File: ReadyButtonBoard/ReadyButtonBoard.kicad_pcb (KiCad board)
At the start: 2 copper layers, 41.9 x 44.5 mm, 7 parts, among them J2 Conn_01x02_Socket

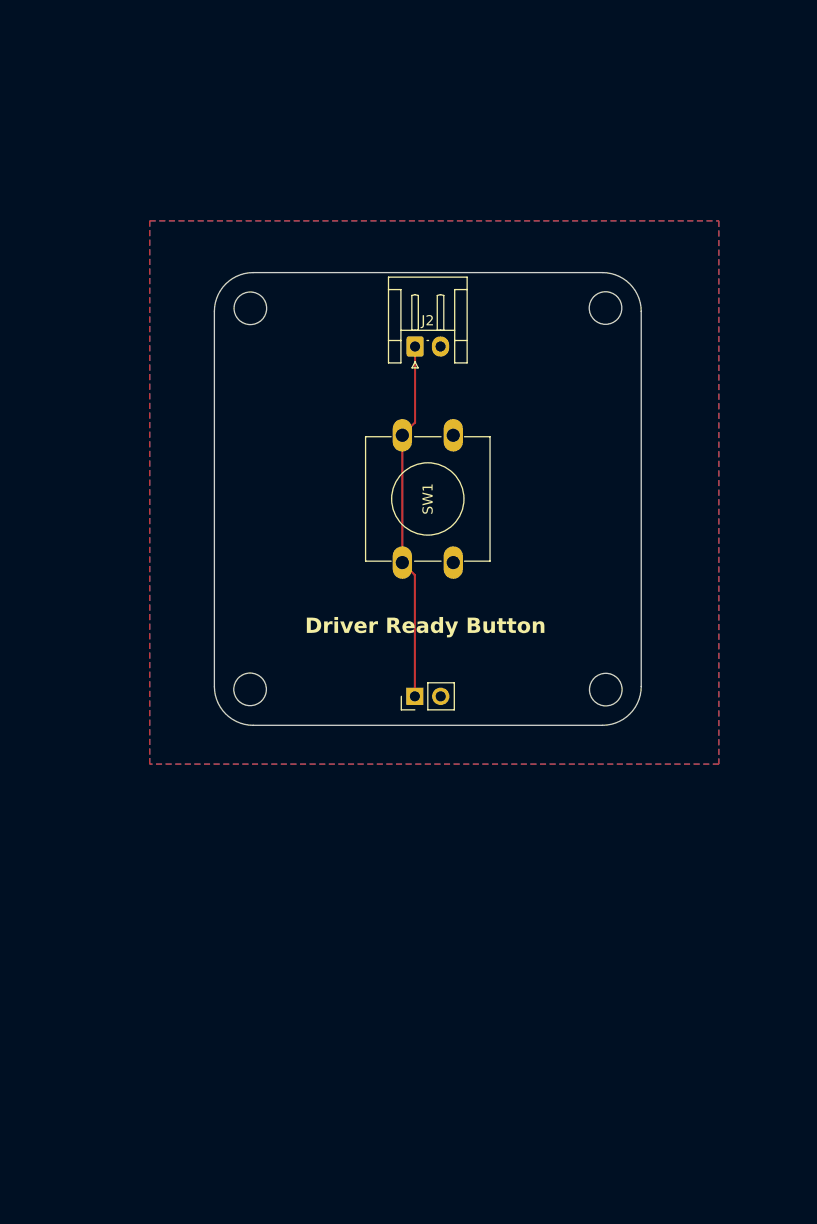
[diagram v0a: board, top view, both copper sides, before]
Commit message: finish ready button board and prod files
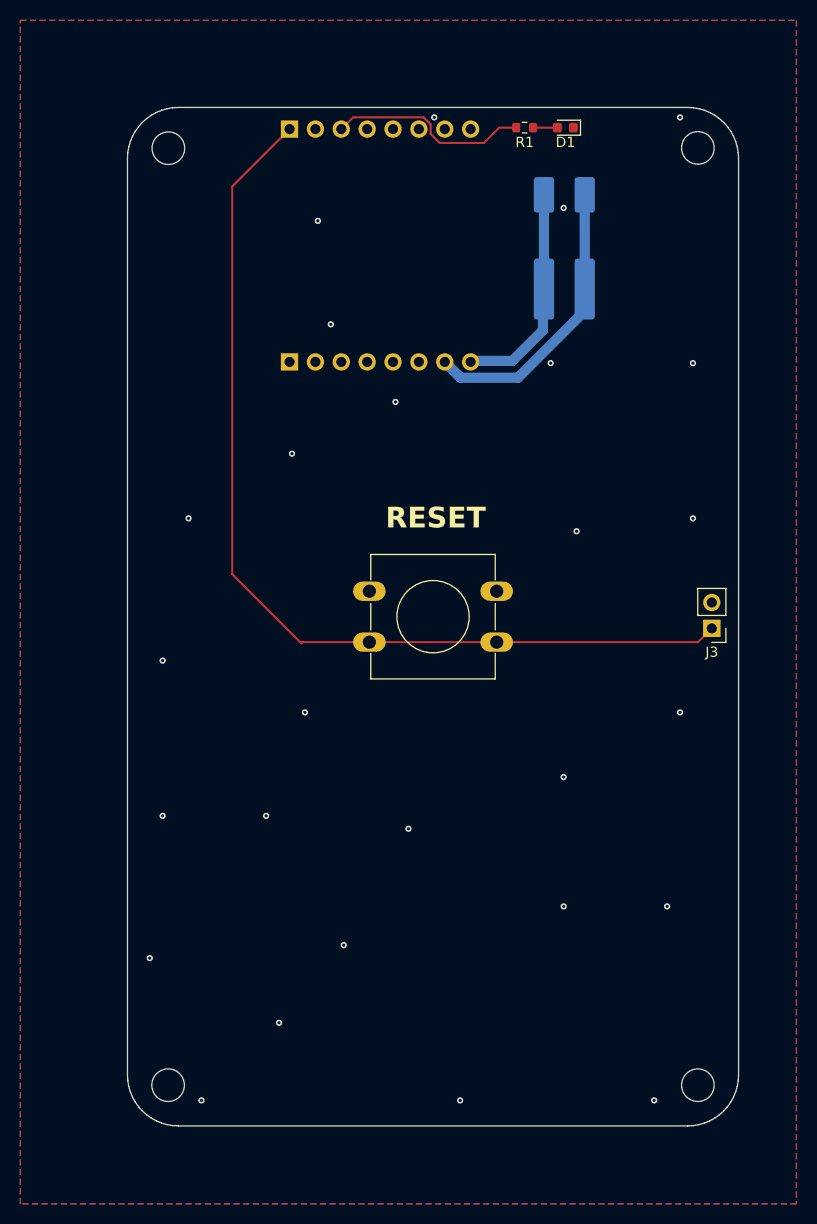
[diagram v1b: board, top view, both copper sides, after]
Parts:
- added D1: Red, LED_SMD:LED_0603_1608Metric, F.Cu at (164.0, 48.0)
- added J3: START, Connector_PinHeader_2.54mm:PinHeader_1x02_P2.54mm_Vertical, F.Cu at (178.4, 97.2)
- added J9: WAGO, WAGO_2060-452_998-404:2060-452_998-404, B.Cu at (163.9, 60.5)
- added R1: 470, Resistor_SMD:R_0603_1608Metric, F.Cu at (160.0, 48.0)
- J1: value ~ -> Conn_01x08_Socket; footprint Connector_PinHeader_2.54mm:PinHeader_1x02_P2.54mm_Vertical -> Connector_PinSocket_2.54mm:PinSocket_1x08_P2.54mm_Vertical; moved to B.Cu
- J2: value Conn_01x02_Socket -> Conn_01x08_Socket; footprint Connector_JST:JST_EH_S2B-EH_1x02_P2.50mm_Horizontal -> Connector_PinSocket_2.54mm:PinSocket_1x08_P2.54mm_Vertical; moved to B.Cu
- SW1: value ~ -> START
- moved J1 57.0 mm to (136.9, 48.1), turned to -90 degrees
- moved H4 39.9 mm to (177.0, 142.0)
- moved H3 39.7 mm to (125.0, 142.0)
- moved H2 18.1 mm to (177.0, 50.0)
- moved H1 17.7 mm to (125.0, 50.0)
- moved SW1 17.4 mm to (144.8, 93.5), turned to 0 degrees
- moved J2 12.4 mm to (136.9, 71.0), turned to -90 degrees
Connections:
- J1 pad 2: GND -> unconnected-(J1-Pin_2-Pad2)
- J2 pad 1: Net-(J1-Pin_1) -> unconnected-(J2-Pin_1-Pad1)
- J2 pad 2: GND -> unconnected-(J2-Pin_2-Pad2)
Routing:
- net Net-(J1-Pin_1): track 35.4 -> 96.5 mm
- net GND: track 0.00 -> 29.9 mm, vias 0 -> 27
- net +5V: track 0.00 -> 23.2 mm
- net Net-(J1-Pin_3): track 0.00 -> 19.9 mm
- net Net-(D1-A): track 0.00 -> 2.39 mm
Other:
- board size 41.9 x 44.5 mm -> 60 x 100 mm
- board text added: "+"
- board text added: "-"
- board text added: "ANTENNA"
- board text added: "Battery Input 5V max!"
- board text added: "Driver Ready/Tapout Board"
- board text added: "RESET"
- board text added: "Vinnie Marco SEMO Combat Robotics 2026"
- board text removed: "Driver Ready Button"
